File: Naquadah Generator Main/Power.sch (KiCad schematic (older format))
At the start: 30 parts, among them U5 AP9101CK6, U6 ECH8695R-TL-W, U8 PAM2423AECADJR

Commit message: Before updating to two switches
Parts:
- J10: renamed from J?; footprint Naquadah_Generator:Power_Mother_Board_Conn -> Naquadah_Generator:Mother_Board_Vert_4_Pin_JST_Conn; symbol Naquadah_Generator:Power_Daughter_Conn -> Naquadah_Generator:Power_Daughter_4_Pin_Conn
- J9: renamed from J?; value Conn_XT -> Power_Conn; footprint (none) -> Naquadah_Generator:Keystone-1042; symbol Connectors_LE:Conn_XT -> Connectors_LE:Power_Conn
- gave numbers to parts that had none: 5
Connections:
- wire segments 126 -> 118
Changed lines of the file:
@@
 	8100 1400 8300 1400
 $Comp
-L Frequently_Used:TestPoint TP?
+L Frequently_Used:TestPoint TP2
 U 1 1 5EDC8A6F
 P 2600 5650
-F 0 "TP?" H 2600 5850 50  0000 C CNN
+F 0 "TP2" H 2600 5850 50  0000 C CNN
 F 1 "TestPoint" H 2500 5400 50  0001 L CNN
 F 2 "Frequently_Used:Pad_2.5-2.5" H 2800 5650 50  0001 C CNN
@@
 	2950 6050 3250 6050
 $Comp
-L Li-ion_5A_Boost_1A_Charge_Protect:R R?
+L Li-ion_5A_Boost_1A_Charge_Protect:R R33
 U 1 1 5EDD5F2C
 P 3500 6050
-F 0 "R?" V 3600 6050 59  0000 L CNN
+F 0 "R33" V 3600 6050 59  0000 L CNN
 F 1 "100" V 3400 6000 59  0000 L CNN
 F 2 "Li-ion 5A Boost 1A Charge Protect:0805_2012Metric_HandSolder" H 3500 6050 50  0001 C CNN
@@
 	2950 5550 3050 5550
 $Comp
-L Li-ion_5A_Boost_1A_Charge_Protect:R R?
+L Li-ion_5A_Boost_1A_Charge_Protect:R R2
 U 1 1 5ED9A5CF
 P 2950 5800
-F 0 "R?" V 2850 5700 59  0000 L CNN
+F 0 "R2" V 2850 5700 59  0000 L CNN
 F 1 "1k" V 3050 5700 59  0000 L CNN
 F 2 "Li-ion 5A Boost 1A Charge Protect:0805_2012Metric_HandSolder" H 2950 5800 50  0001 C CNN
@@
 $EndComp
 $Comp
-L Naquadah_Generator:Power_Daughter_Conn J?
+L Naquadah_Generator:Power_Daughter_4_Pin_Conn J?
 U 1 1 5EDED880
-P 5400 5600
-F 0 "J?" H 5477 5133 50  0000 C CNN
-F 1 "Power_Daughter_Conn" H 5477 5224 50  0000 C CNN
-F 2 "Naquadah_Generator:Power_Mother_Board_Conn" H 5450 4800 50  0001 C CNN
-F 3 "http://www.jst-mfg.com/product/pdf/eng/eSH.pdf" H 5400 5550 50  0001 C CNN
-F 4 "Connector Header Surface Mount 6 position 0.039\" (1.00mm)" H 5450 4700 50  0001 C CNN "Description"
-F 5 "455-1792-1-ND" H 5450 5100 50  0001 C CNN "Digikey Part No."
-F 6 "JST Sales America Inc." H 5450 5000 50  0001 C CNN "Manufacturer Name"
-F 7 "BM06B-SRSS-TB(LF)(SN)" H 5450 4900 50  0001 C CNN "Manufacturer Part No."
-	1    5400 5600
+P 5400 5500
+AR Path="/5EDED880" Ref="J?"  Part="1"
+AR Path="/5EA6751D/5EDED880" Ref="J10"  Part="1"
+F 0 "J10" H 5400 5200 50  0000 C CNN
+F 1 "Power_Daughter_Conn" H 5400 5750 50  0000 C CNN
+F 2 "Naquadah_Generator:Mother_Board_Vert_4_Pin_JST_Conn" H 5450 4700 50  0001 C CNN
+F 3 "http://www.jst-mfg.com/product/pdf/eng/eSH.pdf" H 5400 5450 50  0001 C CNN
+F 4 "Connector Header Surface Mount 6 position 0.039\" (1.00mm)" H 5450 4600 50  0001 C CNN "Description"
+F 5 "455-1792-1-ND" H 5450 5000 50  0001 C CNN "Digikey Part No."
+F 6 "JST Sales America Inc." H 5450 4900 50  0001 C CNN "Manufacturer Name"
+F 7 "BM06B-SRSS-TB(LF)(SN)" H 5450 4800 50  0001 C CNN "Manufacturer Part No."
+	1    5400 5500
 	-1   0    0    1
 $EndComp
 Wire Wire Line
-	5550 5850 5600 5850
+	5550 5550 6100 5550
 Wire Wire Line
-	5600 5850 5600 5800
-Wire Wire Line
-	5600 5750 5550 5750
-Wire Wire Line
-	5550 5650 5600 5650
-Wire Wire Line
-	5600 5650 5600 5600
-Wire Wire Line
-	5600 5550 5550 5550
-Wire Wire Line
-	5600 5600 6100 5600
-Connection ~ 5600 5600
-Wire Wire Line
-	5600 5600 5600 5550
-Wire Wire Line
-	5600 5800 6100 5800
-Connection ~ 5600 5800
-Wire Wire Line
-	5600 5800 5600 5750
+	5550 5650 6100 5650
 Wire Wire Line
 	5550 5450 6100 5450
@@
 Text Label 6100 5450 2    50   ~ 0
 SWITCH
-Text Label 6100 5600 2    50   ~ 0
+Text Label 6100 5550 2    50   ~ 0
 BATT+
-Text Label 6100 5800 2    50   ~ 0
+Text Label 6100 5650 2    50   ~ 0
 GND
 Wire Wire Line
@@
 	1900 5450 2100 5450
 $Comp
-L Connectors_LE:Conn_XT J?
+L Connectors_LE:Power_Conn J9
 U 1 1 5EE056F1
 P 1750 5450
-F 0 "J?" H 1728 5133 50  0000 C CNN
-F 1 "Conn_XT" H 1728 5224 50  0000 C CNN
-F 2 "" H 1750 5450 50  0001 C CNN
+F 0 "J9" H 1750 5250 50  0000 C CNN
+F 1 "Power_Conn" H 1750 5550 50  0000 C CNN
+F 2 "Naquadah_Generator:Keystone-1042" H 1750 5450 50  0001 C CNN
 F 3 "~" H 1750 5450 50  0001 C CNN
 	1    1750 5450
@@
 	2200 5250 2600 5250
 $Comp
-L Frequently_Used:TestPoint TP?
+L Frequently_Used:TestPoint TP1
 U 1 1 5EDB4F62
 P 2600 5150
-F 0 "TP?" H 2600 5450 50  0000 C CNN
+F 0 "TP1" H 2600 5450 50  0000 C CNN
 F 1 "TestPoint" H 2500 4900 50  0001 L CNN
 F 2 "Frequently_Used:Pad_2.5-2.5" H 2800 5150 50  0001 C CNN
@@
 $EndComp
 $Comp
-L Transistor_FET:BSS138 Q?
+L Transistor_FET:BSS138 Q1
 U 1 1 5EDE9E44
 P 3250 5650
-F 0 "Q?" V 3300 5800 50  0000 L CNN
+F 0 "Q1" V 3300 5800 50  0000 L CNN
 F 1 "30V 5A" V 3200 5800 50  0000 L CNN
 F 2 "Naquadah_Generator:SOT-23_Handsoldering" H 3450 5575 50  0001 L CIN

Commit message: Updates
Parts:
- removed D30: RED, Li-ion 5A Boost 1A Charge Protect:LED_0805_2012Metric_HandSolder, symbol Li-ion_5A_Boost_1A_Charge_Protect:LED
- removed R42: 1k, Li-ion 5A Boost 1A Charge Protect:0805_2012Metric_HandSolder, symbol Li-ion_5A_Boost_1A_Charge_Protect:R
- removed W7, W8: 2.5x5.0, Li-ion 5A Boost 1A Charge Protect:Pad_3.0-5.0_w_TH, symbol Li-ion_5A_Boost_1A_Charge_Protect:TestPoint
- added TP10, TP11, TP7, TP8, TP9: TestPoint, Frequently_Used:Pad_2.5-2.5, symbol Frequently_Used:TestPoint
- J10: value Power_Daughter_Conn -> Power Board Conn; footprint Naquadah_Generator:Mother_Board_Vert_4_Pin_JST_Conn -> Naquadah_Generator:Mother_Board_Vert_5_Pin_JST_Conn; symbol Naquadah_Generator:Power_Daughter_4_Pin_Conn -> Naquadah_Generator:Power_Daughter_5_Pin_Conn
- TP1: Name BATT+ -> SWBATT-
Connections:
- net labels added: +5V, MODE, SWBATT-, SWGATE
- wire segments 118 -> 127
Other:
- moved on the sheet: J9, Q1

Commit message: Updates
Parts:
- J10: Digikey Part No. 455-1792-1-ND -> (none); Source (none) -> Digikey; Source Part No. (none) -> 455-1792-1-ND
- TP10, TP11, TP7, TP8, TP9: Description (none) -> None; Manufacturer None -> (none); Manufacturer Name (none) -> None
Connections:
- net labels added: PG1, PG2
- wire segments 127 -> 126
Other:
- moved on the sheet: J10, J9

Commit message: Move libraries and added configuration path.
Moved Li-Ion library to common KiCad library.  Added variables to configuration paths to reference my KiCad libraries.  Moved all 3D components to my common library.
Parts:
- C11, C19: footprint Li-ion 5A Boost 1A Charge Protect:UCD1E471MNL1GS -> Li-ion:UCD1E471MNL1GS; symbol Li-ion_5A_Boost_1A_Charge_Protect:CP1 -> Li-ion_LE:CP1
- C12, C13, C14, C15, C17, C18, C9: footprint Li-ion 5A Boost 1A Charge Protect:0805_2012Metric_HandSolder -> Li-ion:0805_2012Metric_HandSolder; symbol Li-ion_5A_Boost_1A_Charge_Protect:C -> Li-ion_LE:C
- D29: footprint Li-ion 5A Boost 1A Charge Protect:DO-214AC -> Li-ion:DO-214AC; symbol Li-ion_5A_Boost_1A_Charge_Protect:D -> Li-ion_LE:D
- L1: footprint Li-ion 5A Boost 1A Charge Protect:L_MGV0605 -> Li-ion:L_MGV0605; symbol Li-ion_5A_Boost_1A_Charge_Protect:L -> Li-ion_LE:L
- R2, R31, R32, R33, R38, R40, R41: footprint Li-ion 5A Boost 1A Charge Protect:0805_2012Metric_HandSolder -> Li-ion:0805_2012Metric_HandSolder; symbol Li-ion_5A_Boost_1A_Charge_Protect:R -> Li-ion_LE:R
- TP1, TP10, TP11, TP2, TP7, TP8, TP9: footprint Frequently_Used:Pad_2.5-2.5 -> FrequentlyUsed:Pad_2.5-2.5; symbol Frequently_Used:TestPoint -> Frequently_Used_LE:TestPoint
- U5: footprint Li-ion 5A Boost 1A Charge Protect:SOT-23-6 -> Li-ion:SOT-23-6; symbol Li-ion_5A_Boost_1A_Charge_Protect:AP9101CK6 -> Li-ion_LE:AP9101CK6
- U6: footprint Li-ion 5A Boost 1A Charge Protect:SOT65P280X95-8N -> Li-ion:SOT65P280X95-8N; symbol Li-ion_5A_Boost_1A_Charge_Protect:ECH8695R-TL-W_Gates_on_Top -> Li-ion_LE:ECH8695R-TL-W_Gates_on_Top
- U8: footprint Li-ion 5A Boost 1A Charge Protect:PAM2423AECADJR -> Li-ion:PAM2423AECADJR; symbol Li-ion_5A_Boost_1A_Charge_Protect:PAM2423AECADJR -> Li-ion_LE:PAM2423AECADJR

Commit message: PCB Updates
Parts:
- J10: footprint Naquadah_Generator:Mother_Board_Vert_5_Pin_JST_Conn -> Naquadah_Generator:Daughter_Board_Vert_5_Pin_JST_Conn
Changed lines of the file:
@@
 F 0 "J10" H 6400 4750 50  0000 C CNN
 F 1 "Power Board Conn" H 6400 5350 50  0000 C CNN
-F 2 "Naquadah_Generator:Mother_Board_Vert_5_Pin_JST_Conn" H 6450 4250 50  0001 C CNN
+F 2 "Naquadah_Generator:Daughter_Board_Vert_5_Pin_JST_Conn" H 6450 4250 50  0001 C CNN
 F 3 "http://www.jst-mfg.com/product/pdf/eng/eSH.pdf" H 6400 5000 50  0001 C CNN
 F 4 "Connector Header Surface Mount 6 position 0.039\" (1.00mm)" H 6450 4150 50  0001 C CNN "Description"

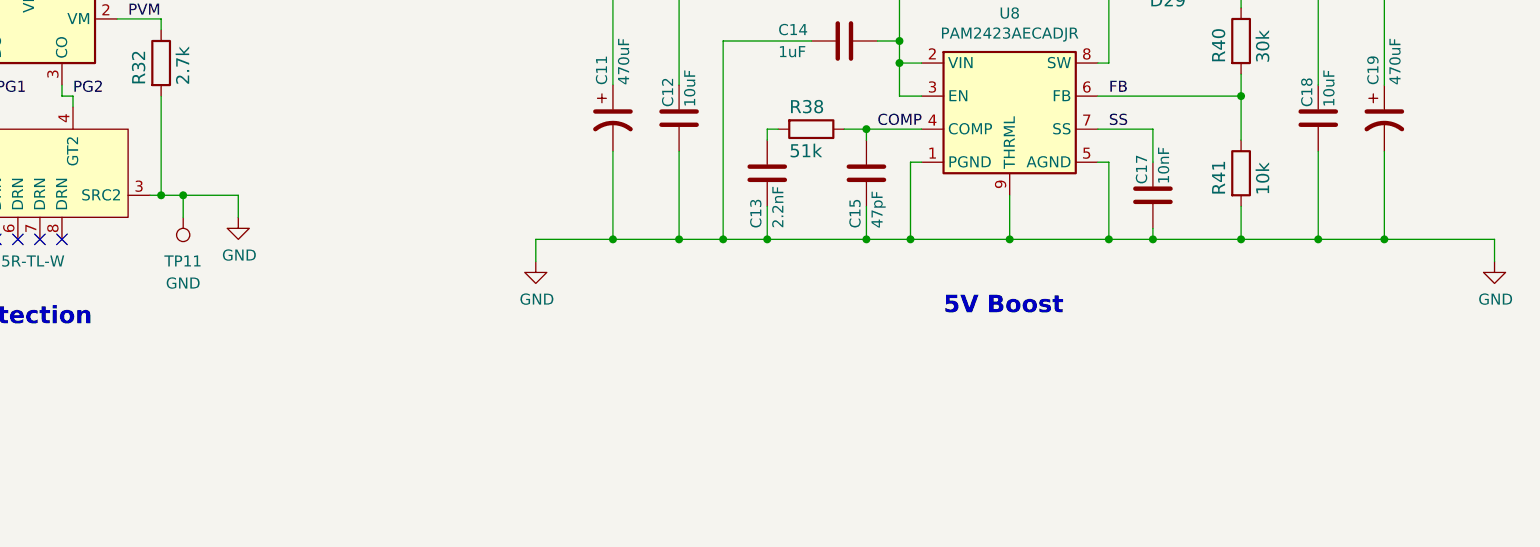
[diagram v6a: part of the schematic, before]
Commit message: Separated digital and analog ground.
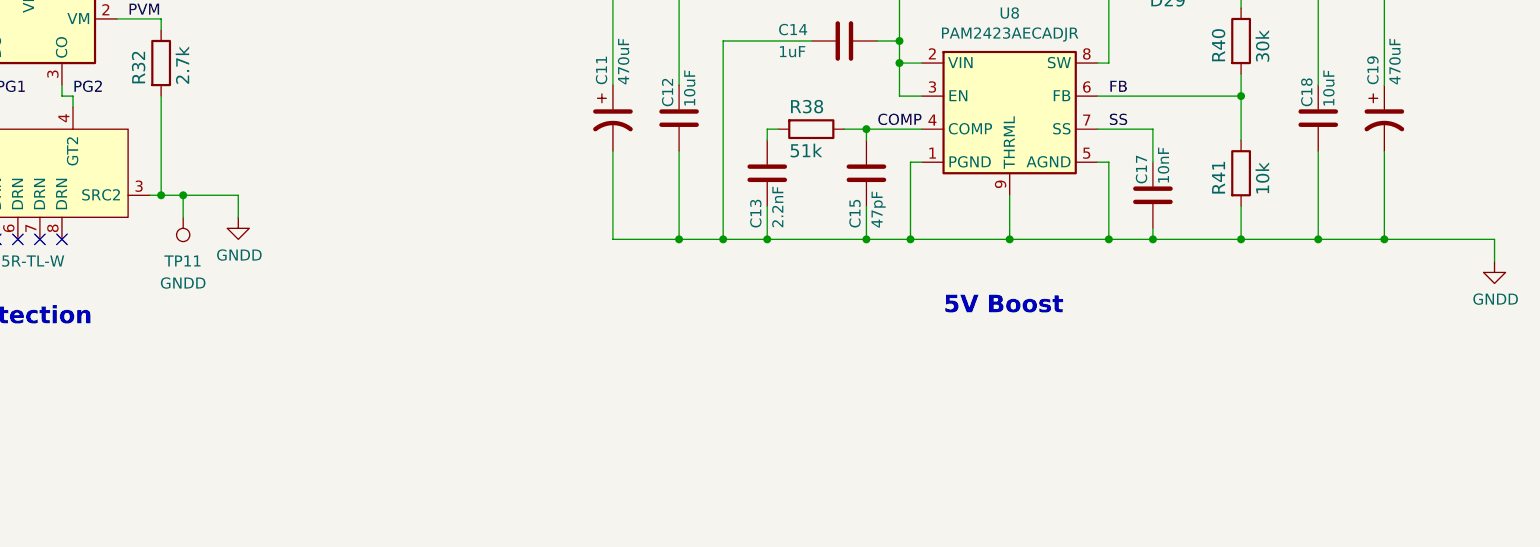
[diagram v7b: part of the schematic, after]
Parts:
- TP11: Name GND -> GNDD
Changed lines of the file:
@@
 	6850 2950 7300 2950
 $Comp
-L power:GND #PWR018
+L Frequently_Used_LE:GNDD #PWR018
 U 1 1 5EC5422D
 P 3800 2850
 F 0 "#PWR018" H 3800 2600 50  0001 C CNN
-F 1 "GND" H 3805 2677 50  0000 C CNN
+F 1 "GNDD" H 3805 2677 50  0000 C CNN
 F 2 "" H 3800 2850 50  0001 C CNN
 F 3 "" H 3800 2850 50  0001 C CNN
@@
 	3800 2750 3800 2850
 $Comp
-L power:GND #PWR019
-U 1 1 5EE79A7F
-P 5150 3050
-F 0 "#PWR019" H 5150 2800 50  0001 C CNN
-F 1 "GND" H 5155 2877 50  0000 C CNN
-F 2 "" H 5150 3050 50  0001 C CNN
-F 3 "" H 5150 3050 50  0001 C CNN
-	1    5150 3050
-	1    0    0    -1
-$EndComp
-$Comp
 L Li-ion_LE:R R31
 U 1 1 5EC910DA
@@
 	1850 1600 1950 1600
 Connection ~ 1950 1600
-Wire Wire Line
-	5150 3050 5150 2950
-Wire Wire Line
-	5150 2950 5500 2950
-Connection ~ 5500 2950
 Text Label 7550 1750 0    50   ~ 0
 SW
@@
 F 2 "FrequentlyUsed:Pad_2.5-2.5" H 3750 2850 50  0001 C CNN
 F 3 "None" H 3750 2850 50  0001 C CNN
-F 4 "GND" H 3550 3150 50  0000 C CNN "Name"
+F 4 "GNDD" H 3550 3150 50  0000 C CNN "Name"
 F 5 "None" H 3545 2495 50  0001 C CNN "Source"
 F 6 "None" H 3545 2495 50  0001 C CNN "Source Part No."
@@
 	9500 1750 9500 1650
 $Comp
-L power:GND #PWR022
+L Frequently_Used_LE:GNDD #PWR022
 U 1 1 5EE6F6B6
 P 9500 3050
 F 0 "#PWR022" H 9500 2800 50  0001 C CNN
-F 1 "GND" H 9505 2877 50  0000 C CNN
+F 1 "GNDD" H 9505 2877 50  0000 C CNN
 F 2 "" H 9500 3050 50  0001 C CNN
 F 3 "" H 9500 3050 50  0001 C CNN

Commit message: Audio update
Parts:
- C11, C19: symbol Li-ion_LE:CP1 -> Li_Ion_LE:CP1
- C12, C13, C14, C15, C17, C18, C9: symbol Li-ion_LE:C -> Li_Ion_LE:C
- D29: symbol Li-ion_LE:D -> Li_Ion_LE:D
- L1: symbol Li-ion_LE:L -> Li_Ion_LE:L
- R2, R41: footprint Li-ion:0805_2012Metric_HandSolder -> Frequently_Used_LE:0805_2012Metric_HandSolder; symbol Li-ion_LE:R -> Li_Ion_LE:R; Source (none) -> Digikey
- R31, R32, R33, R38, R40: footprint Li-ion:0805_2012Metric_HandSolder -> Frequently_Used_LE:0805_2012Metric_HandSolder; symbol Li-ion_LE:R -> Li_Ion_LE:R
- TP1, TP10, TP2, TP7, TP8, TP9: footprint FrequentlyUsed:Pad_2.5-2.5 -> Frequently_Used_LE:Pad_2.5-2.5
- TP11: footprint FrequentlyUsed:Pad_2.5-2.5 -> Frequently_Used_LE:Pad_2.5-2.5; Name GNDD -> DGND
- U5: symbol Li-ion_LE:AP9101CK6 -> Li_Ion_LE:AP9101CK6
- U6: symbol Li-ion_LE:ECH8695R-TL-W_Gates_on_Top -> Li_Ion_LE:ECH8695R-TL-W_Gates_on_Top
- U8: symbol Li-ion_LE:PAM2423AECADJR -> Li_Ion_LE:PAM2423AECADJR
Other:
- note added: "Battery Connector and Power Main Switch"
- note added: "Daughter Board Connector"
- note removed: "Connectors"
- moved on the sheet: J9, Q1, R2, R33
